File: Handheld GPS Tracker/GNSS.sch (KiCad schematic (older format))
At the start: 10 parts

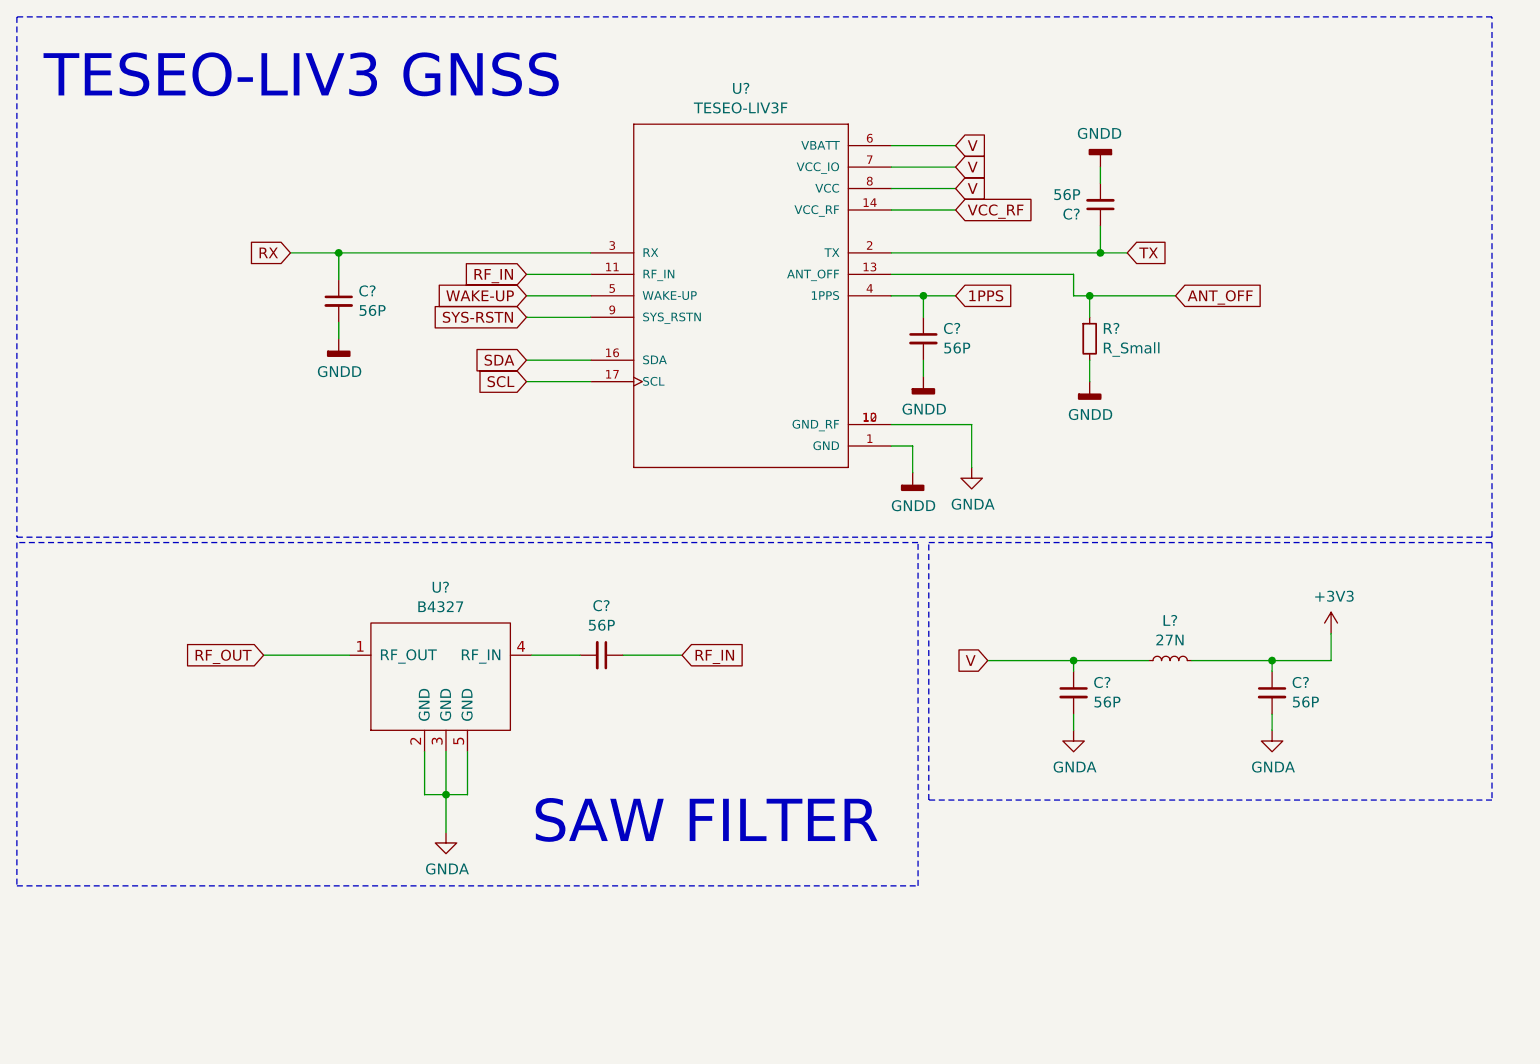
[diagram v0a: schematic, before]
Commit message: Add files via upload
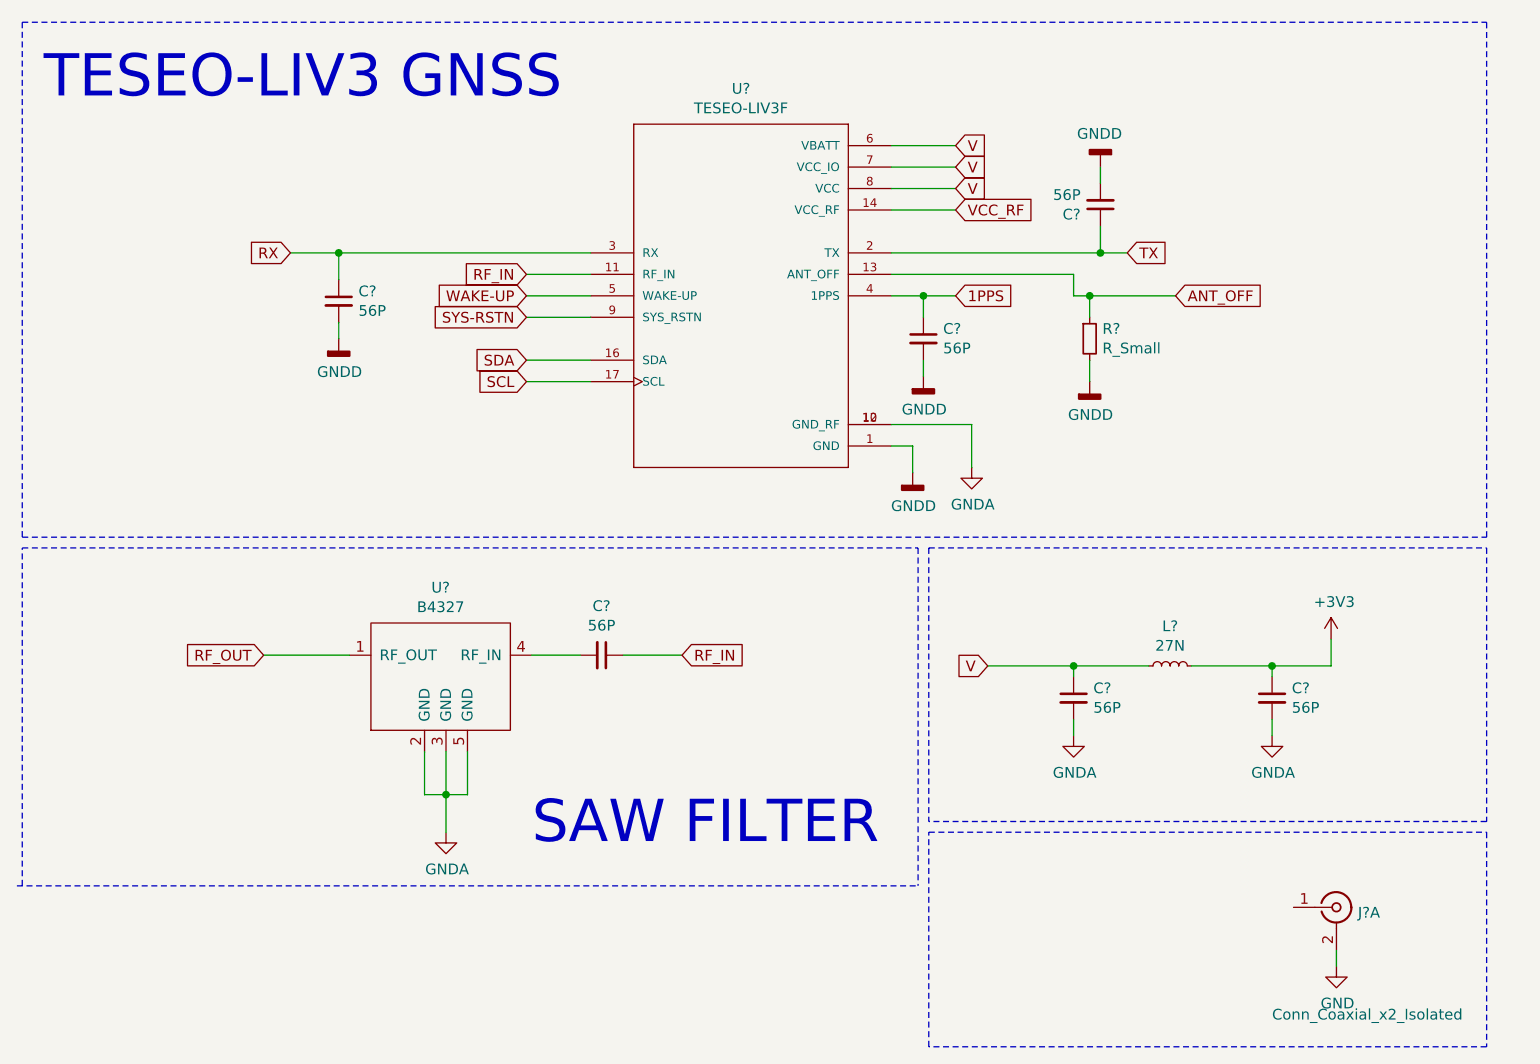
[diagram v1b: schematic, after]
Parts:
- added J?: Conn_Coaxial_x2_Isolated, symbol Connector:Conn_Coaxial_x2_Isolated
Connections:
- new net GND: J?.2 (Ext1)
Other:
- moved on the sheet: C?, L?
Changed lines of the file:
@@
 	1    0    0    -1
 $EndComp
-Wire Notes Line
-	7375 2925 7375 500
-Wire Notes Line
-	7375 500  500  500
-Wire Notes Line
-	500  500  500  2925
-Wire Notes Line
-	500  2925 7375 2925
 $Comp
 L Device:L_Small L?
 U 1 1 5E95725C
-P 5875 3500
-F 0 "L?" V 6060 3500 50  0000 C CNN
-F 1 "27N" V 5969 3500 50  0000 C CNN
-F 2 "" H 5875 3500 50  0001 C CNN
-F 3 "~" H 5875 3500 50  0001 C CNN
-	1    5875 3500
+P 5875 3525
+F 0 "L?" V 6060 3525 50  0000 C CNN
+F 1 "27N" V 5969 3525 50  0000 C CNN
+F 2 "" H 5875 3525 50  0001 C CNN
+F 3 "~" H 5875 3525 50  0001 C CNN
+	1    5875 3525
 	0    -1   -1   0
 $EndComp
@@
 L Device:C_Small C?
 U 1 1 5E957B52
-P 6350 3650
-F 0 "C?" H 6442 3696 50  0000 L CNN
-F 1 "56P" H 6442 3605 50  0000 L CNN
-F 2 "" H 6350 3650 50  0001 C CNN
-F 3 "~" H 6350 3650 50  0001 C CNN
-	1    6350 3650
-	1    0    0    -1
-$EndComp
-Wire Wire Line
-	6350 3550 6350 3500
-Wire Wire Line
-	5975 3500 6350 3500
+P 6350 3675
+F 0 "C?" H 6442 3721 50  0000 L CNN
+F 1 "56P" H 6442 3630 50  0000 L CNN
+F 2 "" H 6350 3675 50  0001 C CNN
+F 3 "~" H 6350 3675 50  0001 C CNN
+	1    6350 3675
+	1    0    0    -1
+$EndComp
+Wire Wire Line
+	6350 3575 6350 3525
+Wire Wire Line
+	5975 3525 6350 3525
 $Comp
 L Device:C_Small C?
 U 1 1 5E958E5C
-P 5425 3650
-F 0 "C?" H 5517 3696 50  0000 L CNN
-F 1 "56P" H 5517 3605 50  0000 L CNN
-F 2 "" H 5425 3650 50  0001 C CNN
-F 3 "~" H 5425 3650 50  0001 C CNN
-	1    5425 3650
-	1    0    0    -1
-$EndComp
-Wire Wire Line
-	5425 3550 5425 3500
-Wire Wire Line
-	5425 3500 5775 3500
-Wire Wire Line
-	5425 3750 5425 3825
+P 5425 3675
+F 0 "C?" H 5517 3721 50  0000 L CNN
+F 1 "56P" H 5517 3630 50  0000 L CNN
+F 2 "" H 5425 3675 50  0001 C CNN
+F 3 "~" H 5425 3675 50  0001 C CNN
+	1    5425 3675
+	1    0    0    -1
+$EndComp
+Wire Wire Line
+	5425 3575 5425 3525
+Wire Wire Line
+	5425 3525 5775 3525
+Wire Wire Line
+	5425 3775 5425 3850
 $Comp
 L power:GNDA #PWR?
 U 1 1 5E95A26B
-P 5425 3825
-F 0 "#PWR?" H 5425 3575 50  0001 C CNN
-F 1 "GNDA" H 5430 3652 50  0000 C CNN
-F 2 "" H 5425 3825 50  0001 C CNN
-F 3 "" H 5425 3825 50  0001 C CNN
-	1    5425 3825
+P 5425 3850
+F 0 "#PWR?" H 5425 3600 50  0001 C CNN
+F 1 "GNDA" H 5430 3677 50  0000 C CNN
+F 2 "" H 5425 3850 50  0001 C CNN
+F 3 "" H 5425 3850 50  0001 C CNN
+	1    5425 3850
 	1    0    0    -1
 $EndComp
@@
 L power:GNDA #PWR?
 U 1 1 5E95A639
-P 6350 3825
-F 0 "#PWR?" H 6350 3575 50  0001 C CNN
-F 1 "GNDA" H 6355 3652 50  0000 C CNN
-F 2 "" H 6350 3825 50  0001 C CNN
-F 3 "" H 6350 3825 50  0001 C CNN
-	1    6350 3825
-	1    0    0    -1
-$EndComp
-Wire Wire Line
-	6350 3750 6350 3825
-Wire Wire Line
-	5425 3500 5025 3500
-Connection ~ 5425 3500
-Text GLabel 5025 3500 0    50   Input ~ 0
+P 6350 3850
+F 0 "#PWR?" H 6350 3600 50  0001 C CNN
+F 1 "GNDA" H 6355 3677 50  0000 C CNN
+F 2 "" H 6350 3850 50  0001 C CNN
+F 3 "" H 6350 3850 50  0001 C CNN
+	1    6350 3850
+	1    0    0    -1
+$EndComp
+Wire Wire Line
+	6350 3775 6350 3850
+Wire Wire Line
+	5425 3525 5025 3525
+Connection ~ 5425 3525
+Text GLabel 5025 3525 0    50   Input ~ 0
 V
 Wire Wire Line
-	6350 3500 6625 3500
-Wire Wire Line
-	6625 3500 6625 3375
-Connection ~ 6350 3500
+	6350 3525 6625 3525
+Wire Wire Line
+	6625 3525 6625 3400
+Connection ~ 6350 3525
 $Comp
 L power:+3V3 #PWR?
 U 1 1 5E95C015
-P 6625 3375
-F 0 "#PWR?" H 6625 3225 50  0001 C CNN
-F 1 "+3V3" H 6640 3548 50  0000 C CNN
-F 2 "" H 6625 3375 50  0001 C CNN
-F 3 "" H 6625 3375 50  0001 C CNN
-	1    6625 3375
+P 6625 3400
+F 0 "#PWR?" H 6625 3250 50  0001 C CNN
+F 1 "+3V3" H 6640 3573 50  0000 C CNN
+F 2 "" H 6625 3400 50  0001 C CNN
+F 3 "" H 6625 3400 50  0001 C CNN
+	1    6625 3400
 	1    0    0    -1
 $EndComp
@@
 Text Notes 625  900  0    197  ~ 0
 TESEO-LIV3 GNSS
-Wire Notes Line
-	7375 2950 7375 4150
-Wire Notes Line
-	7375 4150 4750 4150
-Wire Notes Line
-	4750 4150 4750 2950
+$Comp
+L Connector:Conn_Coaxial_x2_Isolated J?
+U 1 1 5E97048E
+P 6650 4650
+F 0 "J?" H 6750 4625 50  0000 L CNN
+F 1 "Conn_Coaxial_x2_Isolated" H 6350 4150 50  0000 L CNN
+F 2 "" H 6650 4650 50  0001 C CNN
+F 3 " ~" H 6650 4650 50  0001 C CNN
+	1    6650 4650
+	1    0    0    -1
+$EndComp
+Wire Wire Line
+	6650 4850 6650 4925
+$Comp
+L power:GND #PWR?
+U 1 1 5E9732ED
+P 6650 4925
+F 0 "#PWR?" H 6650 4675 50  0001 C CNN
+F 1 "GND" H 6655 4752 50  0000 C CNN
+F 2 "" H 6650 4925 50  0001 C CNN
+F 3 "" H 6650 4925 50  0001 C CNN
+	1    6650 4925
+	1    0    0    -1
+$EndComp
+Text Notes 2900 4375 0    197  ~ 0
+SAW FILTER
+Text GLabel 1650 3475 0    50   Input ~ 0
+RF_OUT
+Wire Wire Line
+	2050 3475 1650 3475
+$Comp
+L power:GNDA #PWR?
+U 1 1 5E97210C
+P 2500 4300
+F 0 "#PWR?" H 2500 4050 50  0001 C CNN
+F 1 "GNDA" H 2505 4127 50  0000 C CNN
+F 2 "" H 2500 4300 50  0001 C CNN
+F 3 "" H 2500 4300 50  0001 C CNN
+	1    2500 4300
+	1    0    0    -1
+$EndComp
+Wire Wire Line
+	2500 4125 2500 4300
+Wire Wire Line
+	2500 4125 2600 4125
+Connection ~ 2500 4125
+Wire Wire Line
+	2500 3925 2500 4125
+Wire Wire Line
+	2600 4125 2600 3925
+Wire Wire Line
+	2400 4125 2500 4125
+Wire Wire Line
+	2400 3925 2400 4125
+Text GLabel 3600 3475 2    50   Input ~ 0
+RF_IN
+Wire Wire Line
+	3325 3475 3600 3475
+Wire Wire Line
+	3125 3475 2900 3475
+$Comp
+L Device:C_Small C?
+U 1 1 5E96E259
+P 3225 3475
+F 0 "C?" V 2996 3475 50  0000 C CNN
+F 1 "56P" V 3087 3475 50  0000 C CNN
+F 2 "" H 3225 3475 50  0001 C CNN
+F 3 "~" H 3225 3475 50  0001 C CNN
+	1    3225 3475
+	0    1    1    0
+$EndComp
 $Comp
 L B4327:B4327 U?
@@
 	1    0    0    -1
 $EndComp
-$Comp
-L Device:C_Small C?
-U 1 1 5E96E259
-P 3225 3475
-F 0 "C?" V 2996 3475 50  0000 C CNN
-F 1 "56P" V 3087 3475 50  0000 C CNN
-F 2 "" H 3225 3475 50  0001 C CNN
-F 3 "~" H 3225 3475 50  0001 C CNN
-	1    3225 3475
-	0    1    1    0
-$EndComp
-Wire Wire Line
-	3125 3475 2900 3475
-Wire Wire Line
-	3325 3475 3600 3475
-Text GLabel 3600 3475 2    50   Input ~ 0
-RF_IN
-Wire Wire Line
-	2400 3925 2400 4125
-Wire Wire Line
-	2400 4125 2500 4125
-Wire Wire Line
-	2600 4125 2600 3925
-Wire Wire Line
-	2500 3925 2500 4125
-Connection ~ 2500 4125
-Wire Wire Line
-	2500 4125 2600 4125
-Wire Wire Line
-	2500 4125 2500 4300
-$Comp
-L power:GNDA #PWR?
-U 1 1 5E97210C
-P 2500 4300
-F 0 "#PWR?" H 2500 4050 50  0001 C CNN
-F 1 "GNDA" H 2505 4127 50  0000 C CNN
-F 2 "" H 2500 4300 50  0001 C CNN
-F 3 "" H 2500 4300 50  0001 C CNN
-	1    2500 4300
-	1    0    0    -1
-$EndComp
-Wire Wire Line
-	2050 3475 1650 3475
-Text GLabel 1650 3475 0    50   Input ~ 0
-RF_OUT
-Wire Notes Line
-	500  2950 500  4550
+Wire Notes Line
+	4700 2975 4700 4550
 Wire Notes Line
 	500  4550 4700 4550
 Wire Notes Line
-	4700 4550 4700 2950
-Wire Notes Line
-	4750 2950 7375 2950
-Wire Notes Line
-	4700 2950 500  2950
-Text Notes 2900 4375 0    197  ~ 0
-SAW FILTER
+	525  4550 525  2975
+Wire Notes Line
+	525  2975 4700 2975
+Wire Notes Line
+	525  525  525  2925
+Wire Notes Line
+	7350 2925 7350 525
+Wire Notes Line
+	525  2925 7350 2925
+Wire Notes Line
+	525  525  7350 525
+Wire Notes Line
+	4750 2975 7350 2975
+Wire Notes Line
+	7350 2975 7350 4250
+Wire Notes Line
+	7350 4250 4750 4250
+Wire Notes Line
+	4750 2975 4750 4250
+Wire Notes Line
+	4750 4300 7350 4300
+Wire Notes Line
+	7350 4300 7350 5300
+Wire Notes Line
+	7350 5300 4750 5300
+Wire Notes Line
+	4750 5300 4750 4300
 $EndSCHEMATC
